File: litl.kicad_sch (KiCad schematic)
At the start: 97 parts

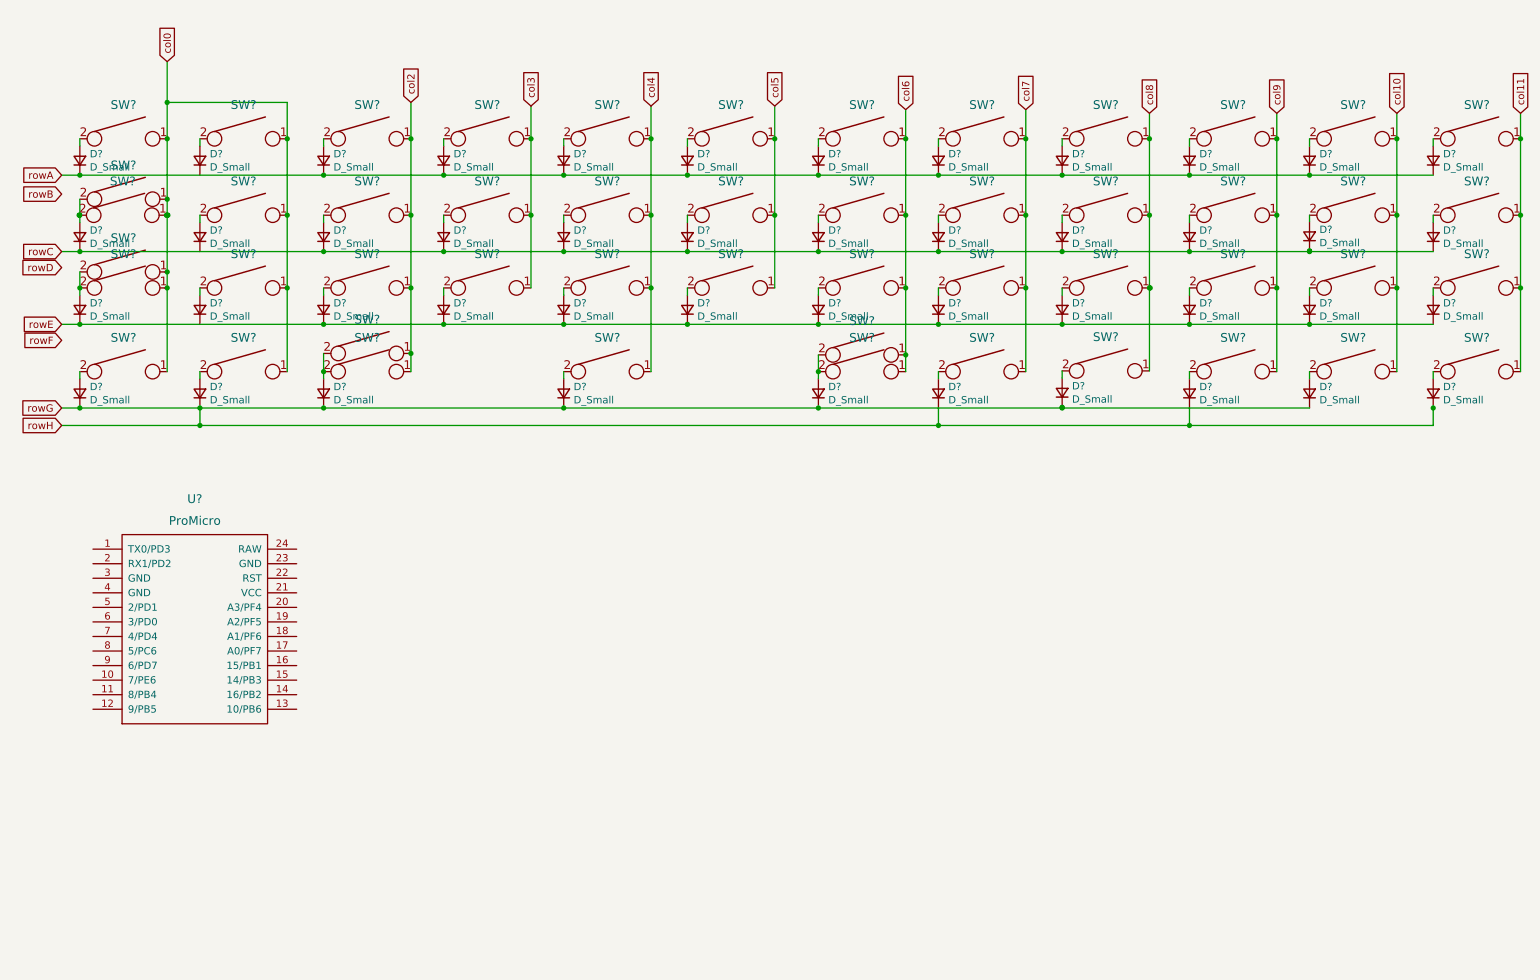
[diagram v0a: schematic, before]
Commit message: Schematic complete
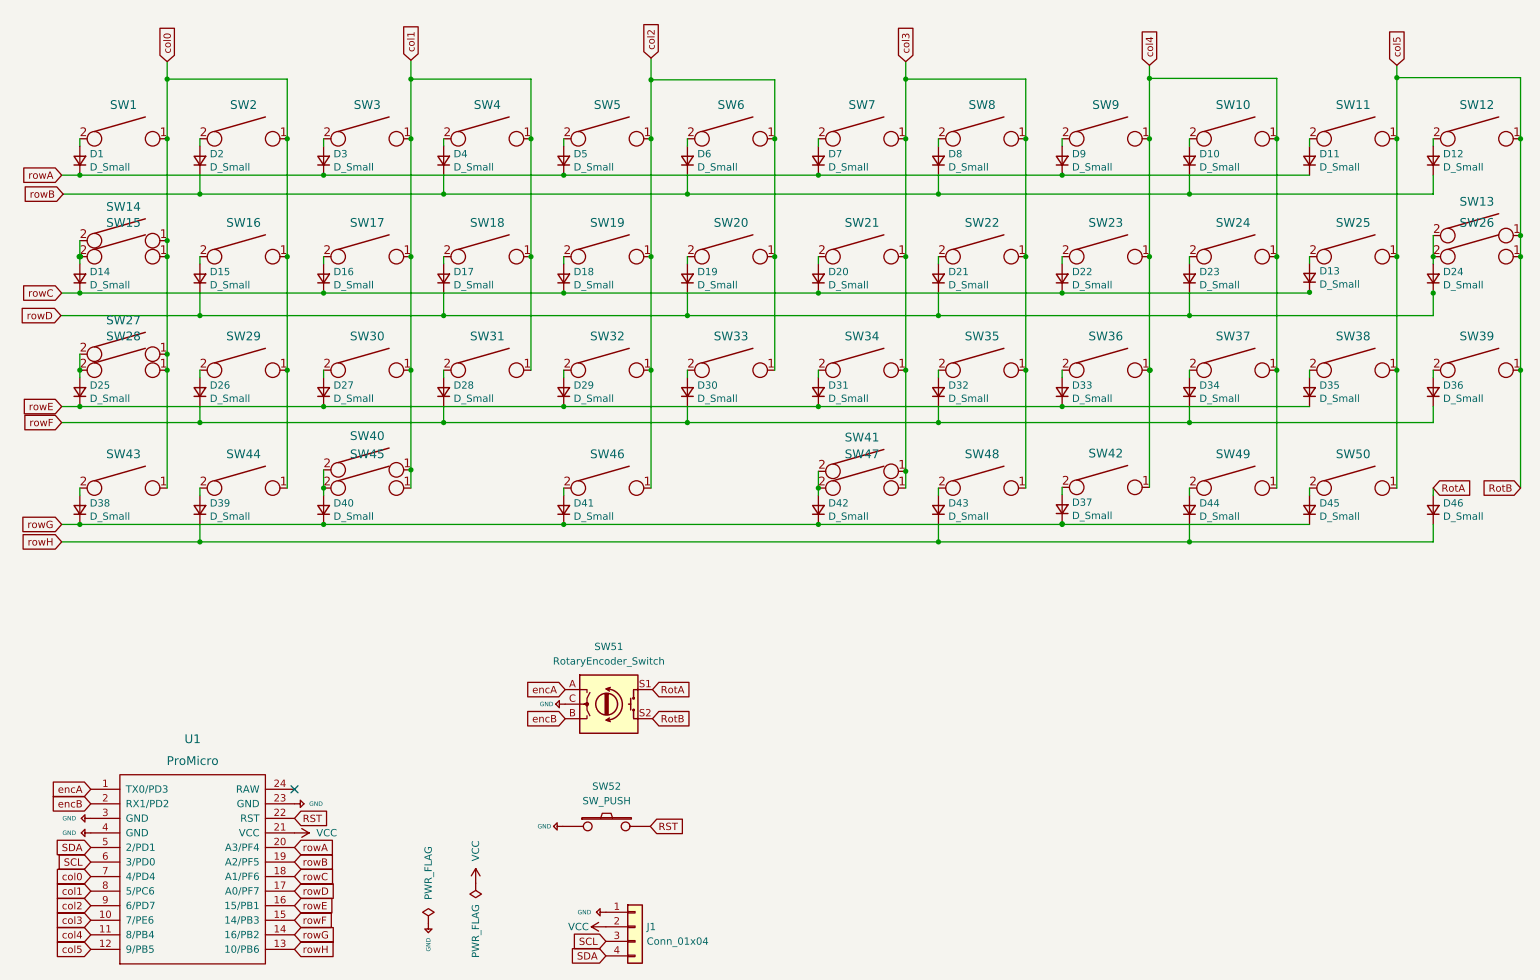
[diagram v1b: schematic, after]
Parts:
- removed SW?: KEYSW, cftkb:SW_Cherry_MX1A_1.25u_PCBNOSCREEN, symbol keyboard_parts:KEYSW
- added J1: Conn_01x04, Connector_PinSocket_2.54mm:PinSocket_1x04_P2.54mm_Vertical, symbol Connector_Generic:Conn_01x04
- added SW13: KEYSW, Button_Switch_Keyboard:SW_Cherry_MX_1.25u_PCB, symbol keyboard_parts:KEYSW
- added SW51: RotaryEncoder_Switch, Keebio-Parts:RotaryEncoder_EC11, symbol Device:RotaryEncoder_Switch
- added SW52: SW_PUSH, Keebio-Parts:SW_Tactile_SPST_Angled_MJTP1117-no-mount, symbol keyboard_parts:SW_PUSH
- D10, D11, D12, D13, D14, D15, D16, D17, D18, D19, D2, D20, D21, D22, D23, D24, D25, D26, D27, D28, D29, D3, D30, D31, D32, D33, D34, D35, D36, D37, D38, D39, D4, D40, D41, D42, D43, D44, D45, D46, D5, D6, D7, D8, D9: renamed from D?; footprint cftkb:D_DO-35_SOD27_P5.08mm_Horizontal -> Keebio-Parts:Diode
- SW1: renamed from SW?; footprint cftkb:SW_Cherry_MX1A_1.50u_PCBNOSCREEN -> Button_Switch_Keyboard:SW_Cherry_MX_1.50u_Plate
- SW10, SW11, SW16, SW17, SW18, SW19, SW2, SW20, SW21, SW22, SW23, SW24, SW25, SW29, SW3, SW30, SW31, SW32, SW33, SW34, SW35, SW36, SW37, SW38, SW4, SW40, SW41, SW44, SW5, SW6, SW7, SW8, SW9: renamed from SW?; footprint cftkb:SW_Cherry_MX1A_1.00u_PCB-NOSCREEN -> Button_Switch_Keyboard:SW_Cherry_MX_1.00u_PCB
- SW12: renamed from SW?; footprint cftkb:SW_Cherry_MX1A_1.50u_PCBNOSCREEN -> Button_Switch_Keyboard:SW_Cherry_MX_1.50u_PCB
- SW14, SW15, SW39: renamed from SW?; footprint cftkb:SW_Cherry_MX1A_1.75u_PCBNOSCREEN -> Button_Switch_Keyboard:SW_Cherry_MX_1.75u_PCB
- SW26, SW27, SW46: renamed from SW?; footprint cftkb:SW_Cherry_MX1A_2.25u_PCBNOSCREEN -> Button_Switch_Keyboard:SW_Cherry_MX_2.25u_PCB
- SW28: renamed from SW?; footprint cftkb:SW_Cherry_MX1A_2.25u_PCBNOSCREEN -> Button_Switch_Keyboard:SW_Cherry_MX_1.25u_PCB
- SW42: renamed from SW?; footprint cftkb:SW_Cherry_MX1A_2.75u_PCB_NOSCREEN -> Button_Switch_Keyboard:SW_Cherry_MX_1.25u_PCB
- SW43: renamed from SW?; footprint cftkb:SW_Cherry_MX1A_1.25u_PCBNOSCREEN -> Button_Switch_Keyboard:SW_Cherry_MX_1.25u_PCB
- SW45, SW50: renamed from SW?; footprint cftkb:SW_Cherry_MX1A_1.00u_PCB-NOSCREEN -> Button_Switch_Keyboard:SW_Cherry_MX_1.25u_PCB
- SW47: renamed from SW?; footprint cftkb:SW_Cherry_MX1A_1.00u_PCB-NOSCREEN -> Button_Switch_Keyboard:SW_Cherry_MX_6.25u_PCB
- SW48: renamed from SW?; footprint cftkb:SW_Cherry_MX1A_2.75u_PCB_NOSCREEN -> Button_Switch_Keyboard:SW_Cherry_MX_2.75u_PCB
- SW49: renamed from SW?; footprint cftkb:SW_Cherry_MX1A_1.25u_PCBNOSCREEN -> Button_Switch_Keyboard:SW_Cherry_MX_1.00u_PCB
- U1: renamed from U?; footprint (none) -> Keebio-Parts:ArduinoProMicro-ZigZag
- gave numbers to parts that had none: 1
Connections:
- net col10 is gone; now on net RotB: SW11.1, SW25.1, SW38.1, SW50.1
- net col11 is gone; now on net RotB: SW12.1, SW26.1, SW39.1
- net col5 is gone; now on net col2: SW20.1, SW33.1, SW6.1
- net col6 is gone; now on net col3: SW21.1, SW34.1, SW41.1, SW47.1, SW7.1
- net col7 is gone; now on net col3: SW22.1, SW35.1, SW48.1, SW8.1
- net col8 is gone; now on net col4: SW23.1, SW36.1, SW42.1, SW9.1
- net col9 is gone; now on net col4: SW10.1, SW24.1, SW37.1, SW49.1
- net col0: now also U1.7 (4/PD4)
- net col2: now also SW19.1, SW32.1, SW46.1, SW5.1, U1.9 (6/PD7); no longer SW17.1, SW3.1, SW30.1, SW40.1, SW45.1
- net col3: now also U1.10 (7/PE6); no longer SW18.1, SW31.1, SW4.1
- net col4: now also U1.11 (8/PB4); no longer SW19.1, SW32.1, SW46.1, SW5.1
- net rowA: now also U1.20 (A3/PF4); no longer D10.1 (K), D12.1 (K), D4.1 (K), D6.1 (K), D8.1 (K)
- net rowB: now also D10.1 (K), D12.1 (K), D2.1 (K), D4.1 (K), D6.1 (K), D8.1 (K), U1.19 (A2/PF5)
- net rowC: now also U1.18 (A1/PF6); no longer D17.1 (K), D19.1 (K), D21.1 (K), D23.1 (K), D24.1 (K)
- net rowD: now also D15.1 (K), D17.1 (K), D19.1 (K), D21.1 (K), D23.1 (K), D24.1 (K), U1.17 (A0/PF7)
- net rowE: now also U1.16 (15/PB1); no longer D28.1 (K), D30.1 (K), D32.1 (K), D34.1 (K), D36.1 (K)
- net rowF: now also D26.1 (K), D28.1 (K), D30.1 (K), D32.1 (K), D34.1 (K), D36.1 (K), U1.15 (14/PB3)
- net rowG: now also U1.14 (16/PB2); no longer D39.1 (K), D43.1 (K), D44.1 (K), D46.1 (K)
- net RotA: now reaches D46.2 (A)
- net RotA: now also SW51.S1
- net at D24.2 (A), SW26.2: now also SW13.2
- net encA: now reaches U1.1 (TX0/PD3)
- net encA: now also SW51.A
- net RotB: now reaches U1.12 (9/PB5)
- net RotB: now also SW13.1, SW51.S2
- net rowH: now reaches U1.13 (10/PB6)
- net rowH: now also D39.1 (K), D43.1 (K), D44.1 (K), D46.1 (K)
- net encB: now reaches U1.2 (RX1/PD2)
- net encB: now also SW51.B
- net VCC: now reaches U1.21 (VCC)
- net VCC: now also J1.2 (Pin_2)
- net RST: now reaches U1.22 (RST)
- net RST: now also SW52.2
- net +5V: now reaches U1.23 (GND)
- net +5V: now also U1.3 (GND), U1.4 (GND), J1.1 (Pin_1), SW51.C, SW52.1
- net SDA: now reaches U1.5 (2/PD1)
- net SDA: now also J1.4 (Pin_4)
- net SCL: now reaches U1.6 (3/PD0)
- net SCL: now also J1.3 (Pin_3)
- net col1: now reaches U1.8 (5/PC6)
- net col1: now also SW17.1, SW18.1, SW3.1, SW30.1, SW31.1, SW4.1, SW40.1, SW45.1
- no-connect marks 0 -> 1
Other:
- moved on the sheet: D13, D14, D15, D16, D17, D18, D19, D20, D21, D22, D23, D24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
